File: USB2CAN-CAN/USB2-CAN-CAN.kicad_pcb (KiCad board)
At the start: 2 copper layers, 50 x 50 mm, 37 parts, among them P1 USB_A, P2 Prog, P3 Term, P4 CONN_01X03, P5 CONN_01X12, P6 CONN_01X12, U1 FT230XS, U2 PIC18F25K80_I/SS, U3 MCP2562

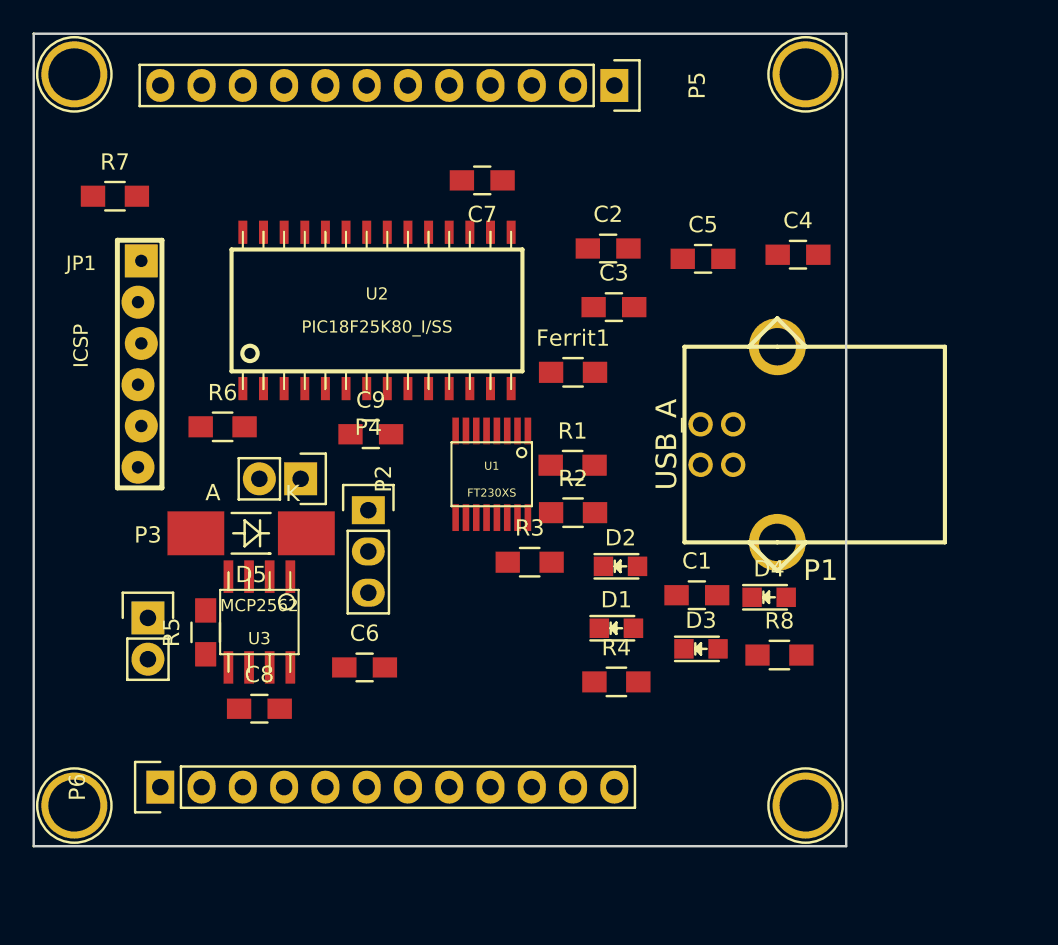
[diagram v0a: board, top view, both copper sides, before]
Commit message: wip
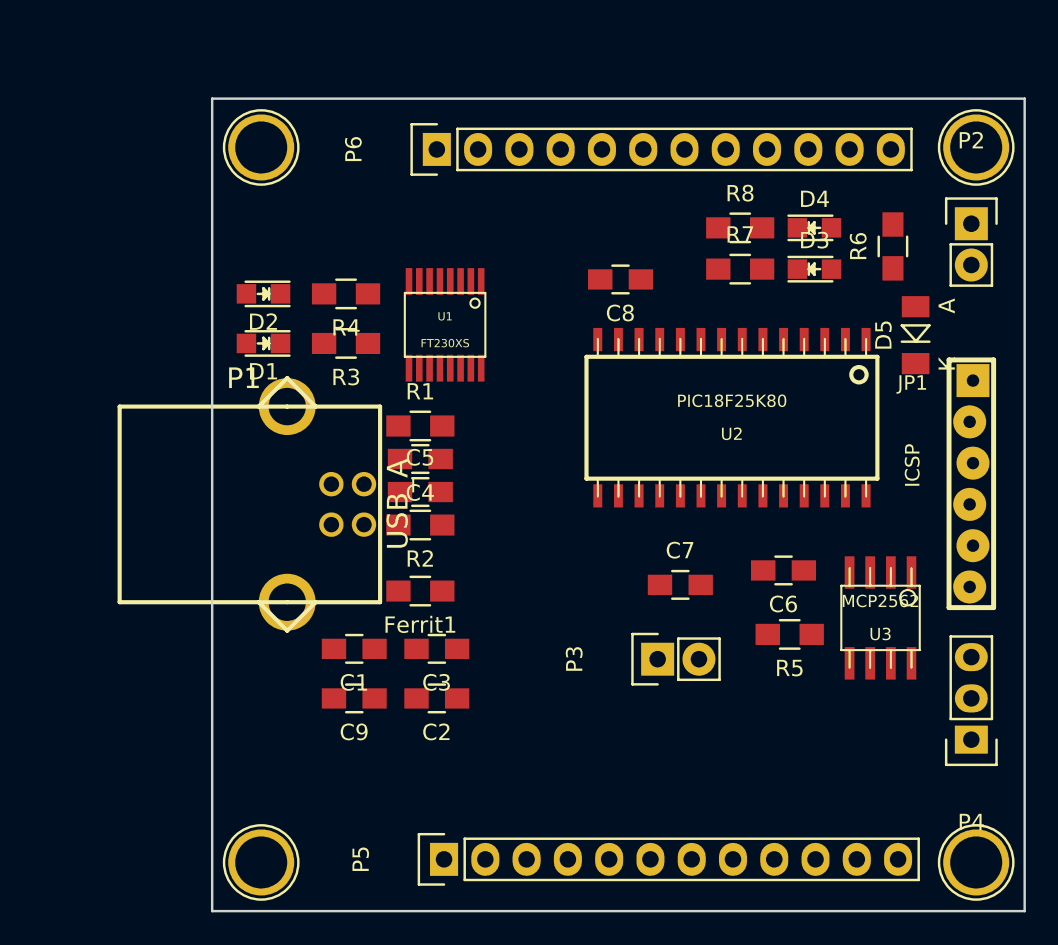
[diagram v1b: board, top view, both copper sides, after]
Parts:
- D5: footprint Diodes_SMD:Diode-MELF_Handsoldering -> Diodes_SMD:MiniMELF_Standard
- P4: value CONN_01X03 -> CAN
- U2: value PIC18F25K80_I/SS -> PIC18F25K80
- moved HLU 73.7 mm to (148.0, 131.0), turned to 180 degrees
- moved HLD 68.7 mm to (148.0, 87.0), turned to 180 degrees
- moved HRU 58.9 mm to (104.0, 131.0), turned to 180 degrees
- moved HRD 52.6 mm to (104.0, 87.0), turned to 180 degrees
- moved JP1 51.7 mm to (147.7, 101.3)
- moved P5 48.8 mm to (115.3, 130.8), turned to 90 degrees
- moved P2 44.2 mm to (147.7, 91.7), turned to 0 degrees
- moved P6 42.8 mm to (114.8, 87.1)
- moved R6 42.7 mm to (142.9, 93.1), turned to 90 degrees
- moved D5 42.7 mm to (144.3, 98.6), turned to 90 degrees
- moved P4 39.7 mm to (147.7, 123.4), turned to 180 degrees
- moved R7 38.7 mm to (133.5, 94.5)
- moved U3 38.2 mm to (142.1, 116.0)
- moved R5 35.9 mm to (136.5, 117.0), turned to 180 degrees
- moved P1 34.9 mm to (103.3, 109.0), turned to 270 degrees
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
